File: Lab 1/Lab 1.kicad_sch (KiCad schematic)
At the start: 66 parts, among them K1 Fujitsu_FTR-LYCA005x, K10 Fujitsu_FTR-LYCA005x, K11 Fujitsu_FTR-LYCA005x, K12 Fujitsu_FTR-LYCA005x, K2 Fujitsu_FTR-LYCA005x, K3 Fujitsu_FTR-LYCA005x, K5 Fujitsu_FTR-LYCA005x, K6 Fujitsu_FTR-LYCA005x, K9 Fujitsu_FTR-LYCA005x, M2 Motor_DC, M4 Motor_DC, M5 Motor_DC, SW1 SW_Push, SW13 SW_SPDT_XKB_DMx-xxxx-1, SW14 SW_SPDT_XKB_DMx-xxxx-1, SW15 STOP, SW16 START, SW17 STOP, SW18 START, SW19 SW_Push, SW2 SW_Push_Open, SW20 SW_SPDT_XKB_DMx-xxxx-1, SW21 SW_Push, SW22 SW_SPDT_XKB_DMx-xxxx-1, SW3 SW_Push, SW4 SW_Push_Open, SW5 SW_Push, SW6 SW_Push

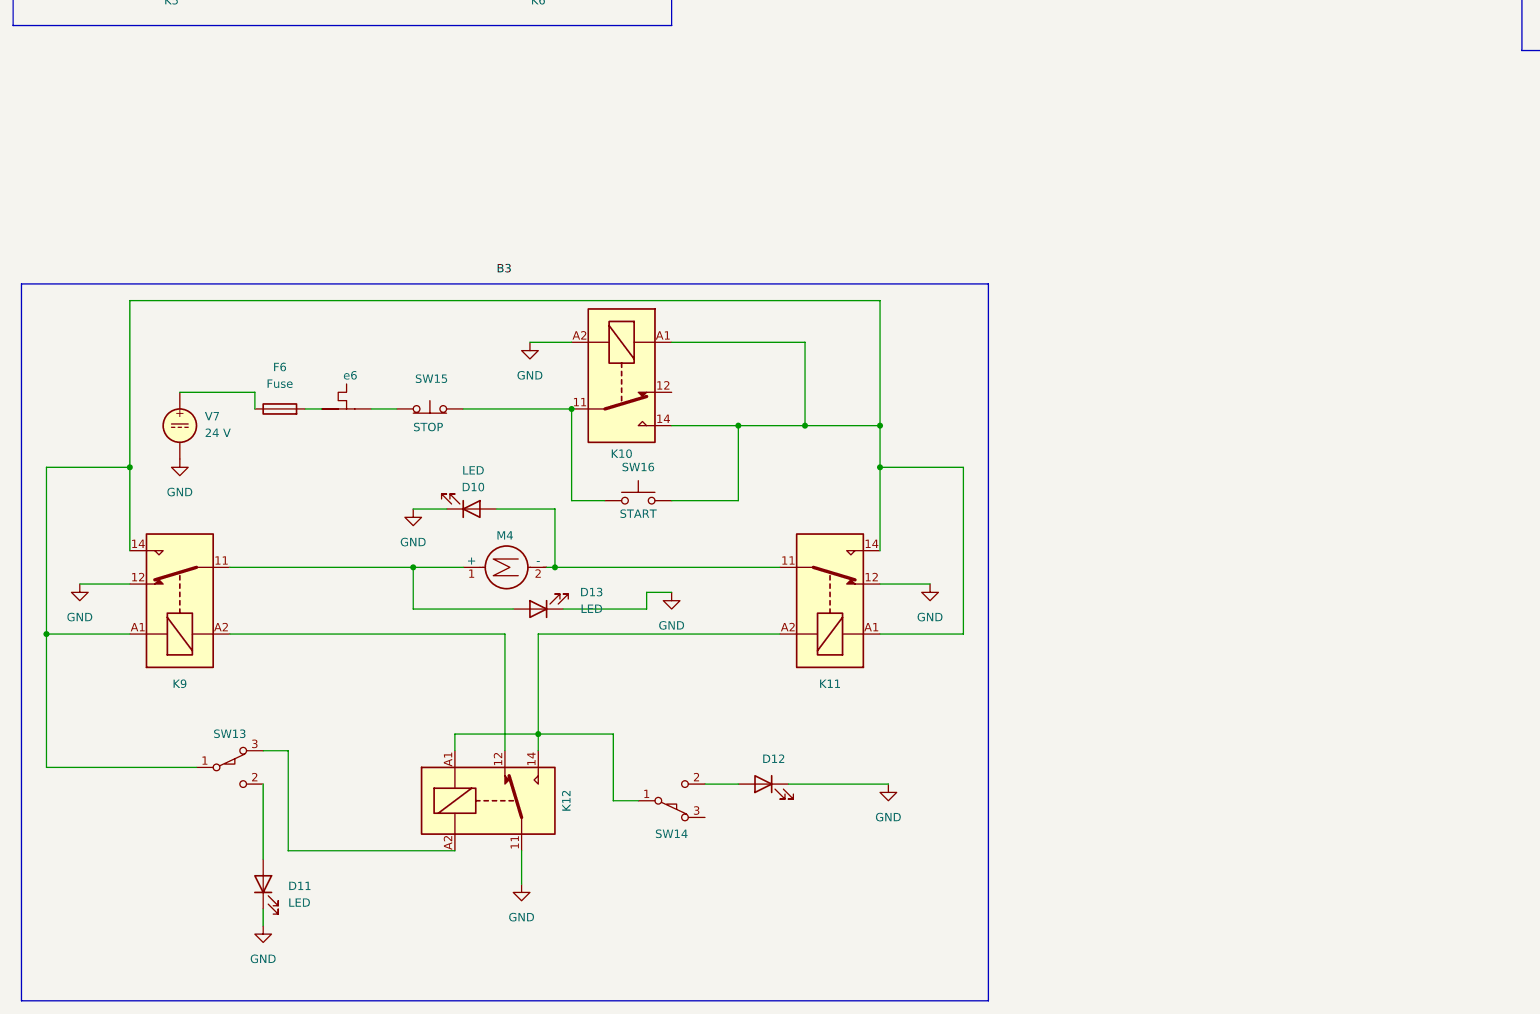
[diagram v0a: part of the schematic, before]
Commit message: Redo B3
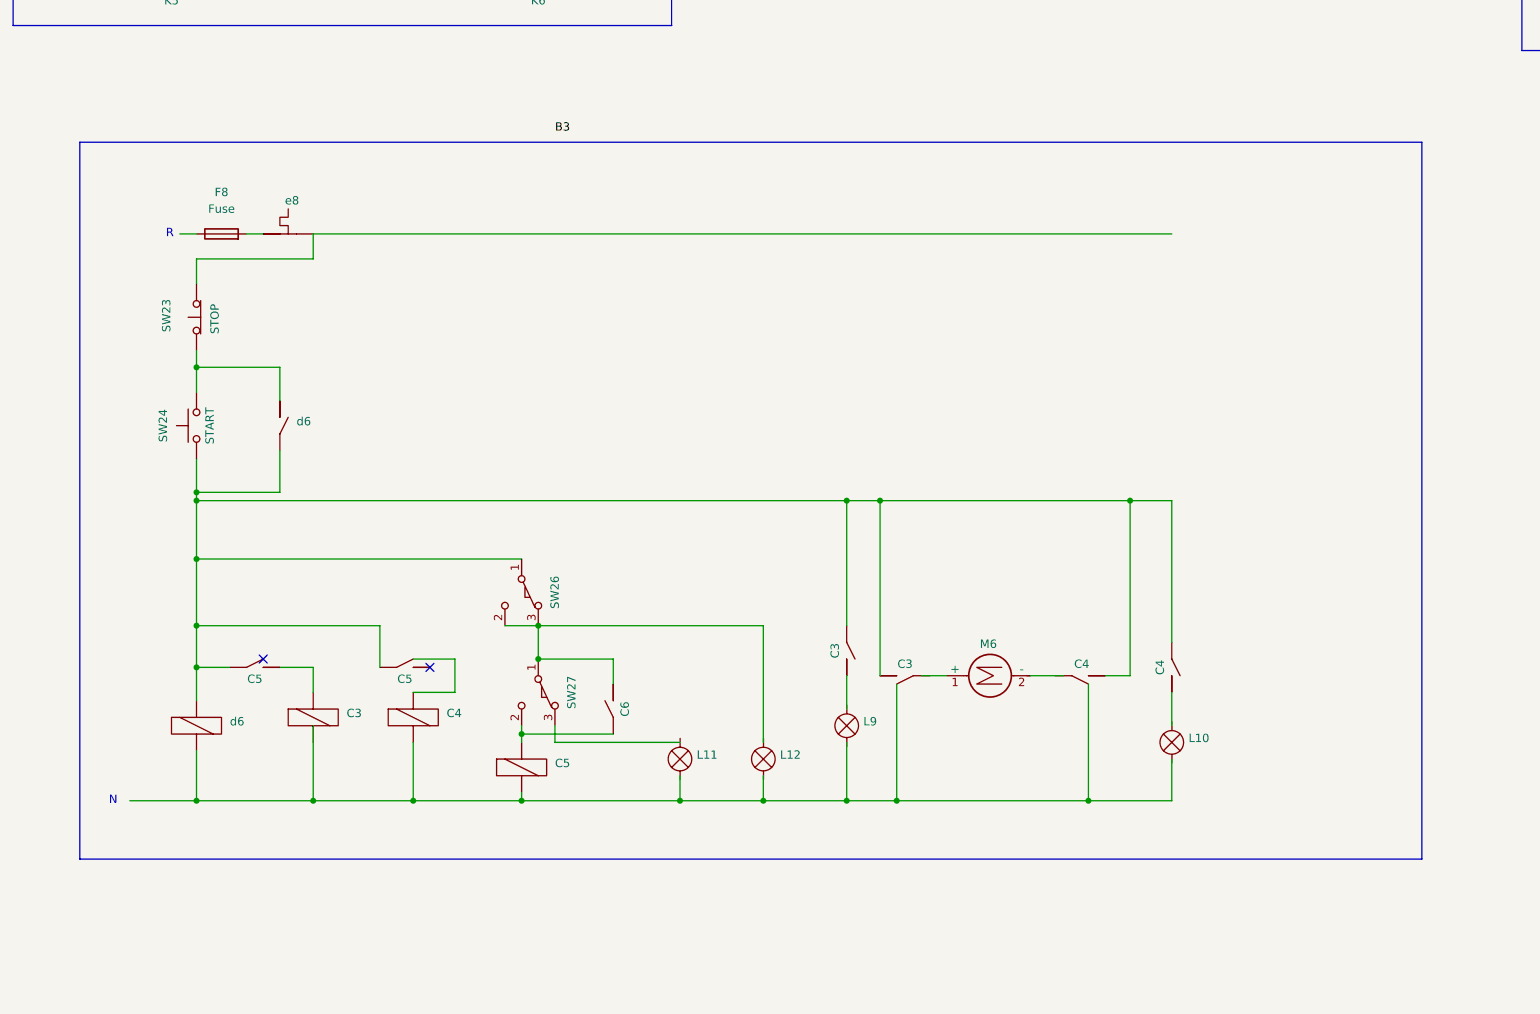
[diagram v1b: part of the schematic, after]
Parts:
- removed D10, D11, D12, D13: LED, symbol Device:LED
- removed F6: Fuse, symbol Device:Fuse
- removed K10, K11, K12, K9: Fujitsu_FTR-LYCA005x, Relay_THT:Relay_SPDT_Fujitsu_FTR-LYCA005x_FormC_Vertical, symbol Relay:Fujitsu_FTR-LYCA005x
- removed M4: Motor_DC, symbol Motor:Motor_DC
- removed SW13, SW14: SW_SPDT_XKB_DMx-xxxx-1, symbol Switch:SW_SPDT_XKB_DMx-xxxx-1
- removed SW15: STOP, symbol Switch:SW_Push_Open
- removed SW16: START, symbol Switch:SW_Push
- removed V7: 24 V, symbol Simulation_SPICE:VDC
- removed e6: ~, symbol relay_contact:Thermal_Contact_NC
- added C3, C4, C5, d6: ~, symbol relay_coil:Relay_coil
- added C3 (x2), C4 (x2), C5 (x2), C6, d6: ~, symbol relay_contact:Relay_contact
- added F8: Fuse, symbol Device:Fuse
- added L10, L11, L12, L9: ~, symbol Indicator:Indicator
- added M6: Motor_DC, symbol Motor:Motor_DC
- added SW23: STOP, symbol Switch:SW_Push_Open
- added SW24: START, symbol Switch:SW_Push
- added SW26, SW27: SW_SPDT_XKB_DMx-xxxx-1, symbol Switch:SW_SPDT_XKB_DMx-xxxx-1
- added e8: ~, symbol relay_contact:Thermal_Contact_NC
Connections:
- new net: SW26.2 (B), SW26.3 (C), SW27.1 (A)
- new net: SW23.1 (A), SW24.2
- new net: SW24.1, SW26.1 (A)
- no-connect marks 0 -> 2
